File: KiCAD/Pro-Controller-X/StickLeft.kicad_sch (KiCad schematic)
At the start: 2 parts, among them J1 Conn_01x05_Pin

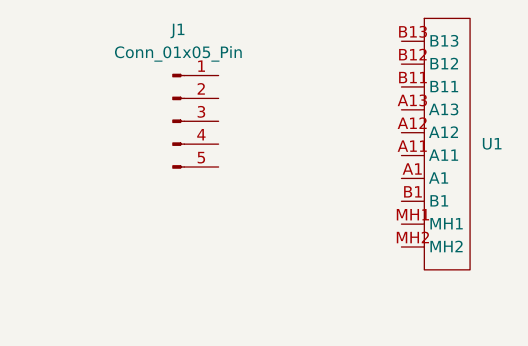
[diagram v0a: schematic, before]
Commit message: Joystick Boards done
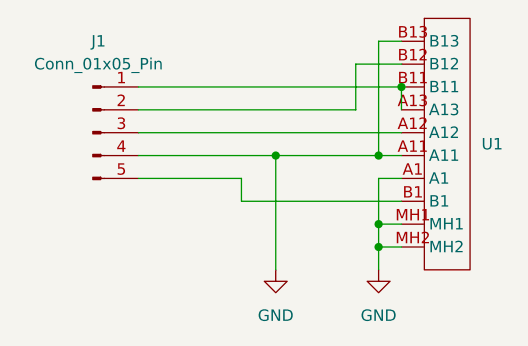
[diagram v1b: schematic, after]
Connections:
- net at J1.1 (Pin_1): now also U1.A13, U1.B11
- net at J1.2 (Pin_2): now also U1.B12
- net at J1.3 (Pin_3): now also U1.A12
- net GND: now reaches J1.4 (Pin_4)
- net GND: now also U1.A1, U1.A11, U1.B13, U1.MH1, U1.MH2
- net at J1.5 (Pin_5): now also U1.B1
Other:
- moved on the sheet: J1
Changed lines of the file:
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@@
 (kicad_sch (version 20230121) (generator eeschema)
   (paper "A2")
-  (symbol (lib_id "Connector:Conn_01x05_Pin") (at 243.84 194.31 0) (unit 1)
+  (junction (at 266.7 198.12) (diameter 0) (color 0 0 0 0)
+  )
+  (junction (at 266.7 208.28) (diameter 0) (color 0 0 0 0)
+  )
+  (junction (at 266.7 205.74) (diameter 0) (color 0 0 0 0)
+  )
+  (junction (at 269.24 190.5) (diameter 0) (color 0 0 0 0)
+  )
+  (junction (at 255.27 198.12) (diameter 0) (color 0 0 0 0)
+  )
+  (wire (pts (xy 269.24 190.5) (xy 269.24 193.04))
+    (stroke (width 0) (type default))
+  )
+  (wire (pts (xy 266.7 205.74) (xy 266.7 208.28))
+    (stroke (width 0) (type default))
+  )
+  (wire (pts (xy 269.24 187.96) (xy 264.16 187.96))
+    (stroke (width 0) (type default))
+  )
+  (wire (pts (xy 266.7 208.28) (xy 266.7 210.82))
+    (stroke (width 0) (type default))
+  )
+  (wire (pts (xy 251.46 200.66) (xy 251.46 203.2))
+    (stroke (width 0) (type default))
+  )
+  (wire (pts (xy 266.7 205.74) (xy 269.24 205.74))
+    (stroke (width 0) (type default))
+  )
+  (wire (pts (xy 240.03 195.58) (xy 269.24 195.58))
+    (stroke (width 0) (type default))
+  )
+  (wire (pts (xy 264.16 187.96) (xy 264.16 193.04))
+    (stroke (width 0) (type default))
+  )
+  (wire (pts (xy 266.7 198.12) (xy 269.24 198.12))
+    (stroke (width 0) (type default))
+  )
+  (wire (pts (xy 240.03 190.5) (xy 269.24 190.5))
+    (stroke (width 0) (type default))
+  )
+  (wire (pts (xy 269.24 203.2) (xy 251.46 203.2))
+    (stroke (width 0) (type default))
+  )
+  (wire (pts (xy 255.27 198.12) (xy 266.7 198.12))
+    (stroke (width 0) (type default))
+  )
+  (wire (pts (xy 240.03 198.12) (xy 255.27 198.12))
+    (stroke (width 0) (type default))
+  )
+  (wire (pts (xy 266.7 208.28) (xy 269.24 208.28))
+    (stroke (width 0) (type default))
+  )
+  (wire (pts (xy 269.24 200.66) (xy 266.7 200.66))
+    (stroke (width 0) (type default))
+  )
+  (wire (pts (xy 266.7 200.66) (xy 266.7 205.74))
+    (stroke (width 0) (type default))
+  )
+  (wire (pts (xy 264.16 193.04) (xy 240.03 193.04))
+    (stroke (width 0) (type default))
+  )
+  (wire (pts (xy 240.03 200.66) (xy 251.46 200.66))
+    (stroke (width 0) (type default))
+  )
+  (wire (pts (xy 269.24 185.42) (xy 266.7 185.42))
+    (stroke (width 0) (type default))
+  )
+  (wire (pts (xy 266.7 185.42) (xy 266.7 198.12))
+    (stroke (width 0) (type default))
+  )
+  (wire (pts (xy 255.27 198.12) (xy 255.27 210.82))
+    (stroke (width 0) (type default))
+  )
+  (symbol (lib_id "Connector:Conn_01x05_Pin") (at 234.95 195.58 0) (unit 1)
     (in_bom yes) (on_board yes) (dnp no) (fields_autoplaced)
-    (property "Reference" "J1" (at 244.475 184.15 0)
+    (property "Reference" "J1" (at 235.585 185.42 0)
       (effects (font (size 1.27 1.27)))
     )
-    (property "Value" "Conn_01x05_Pin" (at 244.475 186.69 0)
+    (property "Value" "Conn_01x05_Pin" (at 235.585 187.96 0)
       (effects (font (size 1.27 1.27)))
     )
-    (property "Footprint" "Connector_PinHeader_2.54mm:PinHeader_1x05_P2.54mm_Horizontal" (at 243.84 194.31 0)
+    (property "Footprint" "Connector_PinHeader_2.54mm:PinHeader_1x05_P2.54mm_Horizontal" (at 234.95 195.58 0)
       (effects (font (size 1.27 1.27)) hide)
     )
-    (property "Datasheet" "~" (at 243.84 194.31 0)
+    (property "Datasheet" "~" (at 234.95 195.58 0)
       (effects (font (size 1.27 1.27)) hide)
     )
@@
         (path "/40a7657d-c4d7-4ebc-b606-0c6932d6f433"
           (reference "J1") (unit 1)
+        )
+      )
+    )
+  )
+  (symbol (lib_id "power:GND") (at 266.7 210.82 0) (unit 1)
+    (in_bom yes) (on_board yes) (dnp no) (fields_autoplaced)
+    (property "Reference" "#PWR01" (at 266.7 217.17 0)
+      (effects (font (size 1.27 1.27)) hide)
+    )
+    (property "Value" "GND" (at 266.7 215.9 0)
+      (effects (font (size 1.27 1.27)))
+    )
+    (property "Footprint" "" (at 266.7 210.82 0)
+      (effects (font (size 1.27 1.27)) hide)
+    )
+    (property "Datasheet" "" (at 266.7 210.82 0)
+      (effects (font (size 1.27 1.27)) hide)
+    )
+    (pin "1")
+    (instances
+      (project "StickLeft"
+        (path "/40a7657d-c4d7-4ebc-b606-0c6932d6f433"
+          (reference "#PWR01") (unit 1)
         )
       )
@@
         )
       )
+    )
+  )
+  (symbol (lib_id "power:GND") (at 255.27 210.82 0) (unit 1)
+    (in_bom yes) (on_board yes) (dnp no) (fields_autoplaced)
+    (property "Reference" "#PWR02" (at 255.27 217.17 0)
+      (effects (font (size 1.27 1.27)) hide)
+    )
+    (property "Value" "GND" (at 255.27 215.9 0)
+      (effects (font (size 1.27 1.27)))
+    )
+    (property "Footprint" "" (at 255.27 210.82 0)
+      (effects (font (size 1.27 1.27)) hide)
+    )
+    (property "Datasheet" "" (at 255.27 210.82 0)
+      (effects (font (size 1.27 1.27)) hide)
+    )
+    (pin "1")
+    (instances
+      (project "StickLeft"
+        (path "/40a7657d-c4d7-4ebc-b606-0c6932d6f433"
+          (reference "#PWR02") (unit 1)
+        )
+      )
